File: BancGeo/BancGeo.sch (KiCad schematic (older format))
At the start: 102 parts

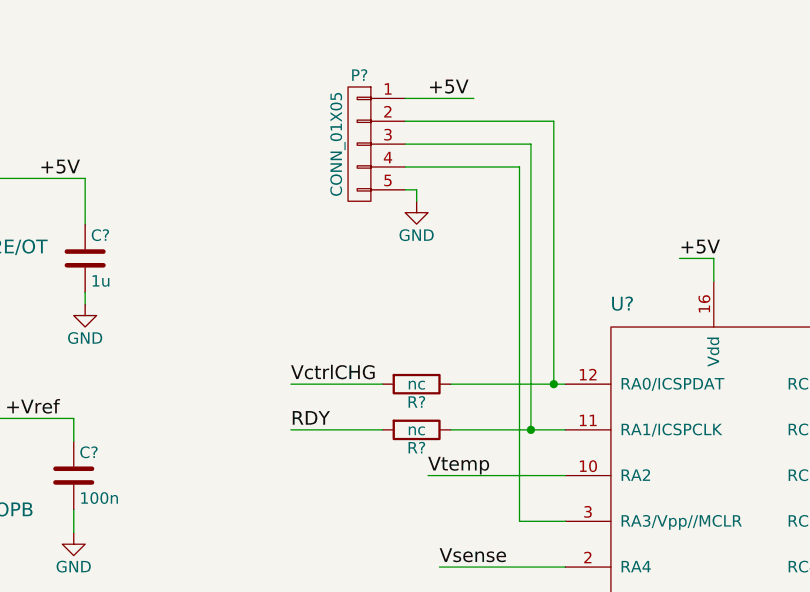
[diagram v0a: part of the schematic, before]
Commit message: Update layout
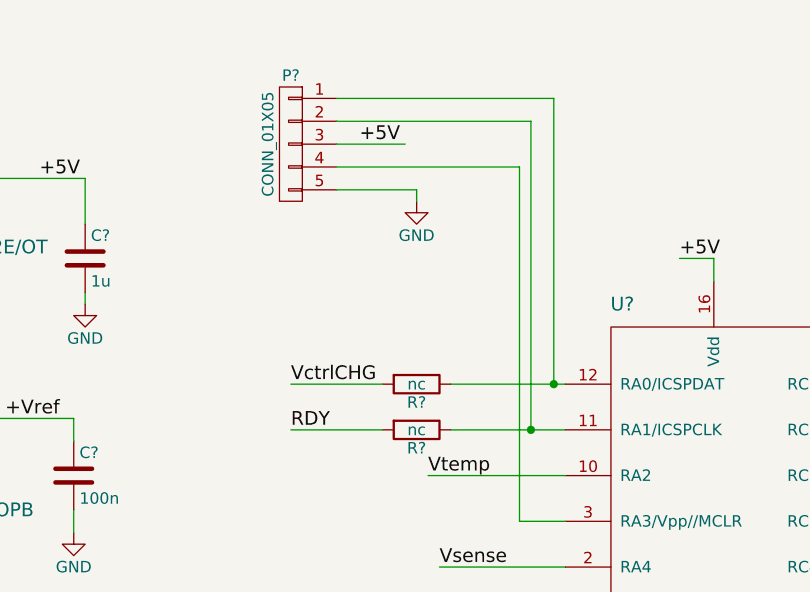
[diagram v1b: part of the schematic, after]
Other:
- moved on the sheet: P?
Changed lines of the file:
@@
 LIBS:contrib
 LIBS:valves
-LIBS:IDBox
 LIBS:BancGeo-cache
+LIBS:YameLib
 EELAYER 25 0
 EELAYER END
@@
 L CONN_01X05 P?
 U 1 1 56BBEC48
-P 6050 1100
-F 0 "P?" H 6050 1400 50  0000 C CNN
-F 1 "CONN_01X05" V 6150 1100 50  0000 C CNN
-F 2 "" H 6050 1100 60  0000 C CNN
-F 3 "" H 6050 1100 60  0000 C CNN
-	1    6050 1100
+P 5750 1100
+F 0 "P?" H 5750 1400 50  0000 C CNN
+F 1 "CONN_01X05" V 5850 1100 50  0000 C CNN
+F 2 "" H 5750 1100 60  0000 C CNN
+F 3 "" H 5750 1100 60  0000 C CNN
+	1    5750 1100
 	-1   0    0    -1
 $EndComp
-Text Label 6350 900  0    60   ~ 0
+Text Label 6050 1100 0    60   ~ 0
 +5V
 $Comp
@@
 	5750 2150 6150 2150
 Wire Wire Line
-	6250 900  6550 900
-Wire Wire Line
-	6250 1300 6300 1300
+	5950 1100 6250 1100
+Wire Wire Line
+	5950 1300 6300 1300
 Wire Wire Line
 	6300 1300 6300 1350
 Wire Wire Line
-	6250 1000 6900 1000
-Wire Wire Line
-	6900 1000 6900 2150
+	6900 900  6900 2150
 Connection ~ 6900 2150
 Wire Wire Line
 	6450 2350 6950 2350
 Wire Wire Line
-	6800 2350 6800 1100
-Wire Wire Line
-	6800 1100 6250 1100
-Wire Wire Line
-	6250 1200 6750 1200
+	6800 1000 6800 2350
 Wire Wire Line
 	6750 1200 6750 2750
@@
 	12550 9300 12550 9250
 Connection ~ 12550 9250
+Wire Wire Line
+	5950 1200 6750 1200
+Wire Wire Line
+	6800 1000 5950 1000
+Wire Wire Line
+	5950 900  6900 900
 $EndSCHEMATC
